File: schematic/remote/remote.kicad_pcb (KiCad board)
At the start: 2 copper layers, 14 parts, among them J1 Conn_01x05_Male, J2 Joystick_Left, J3 Joystick_Right, J4 Micro-Power-IN, J5 NRF-Power, U1 ARDUINO_PRO_MINI

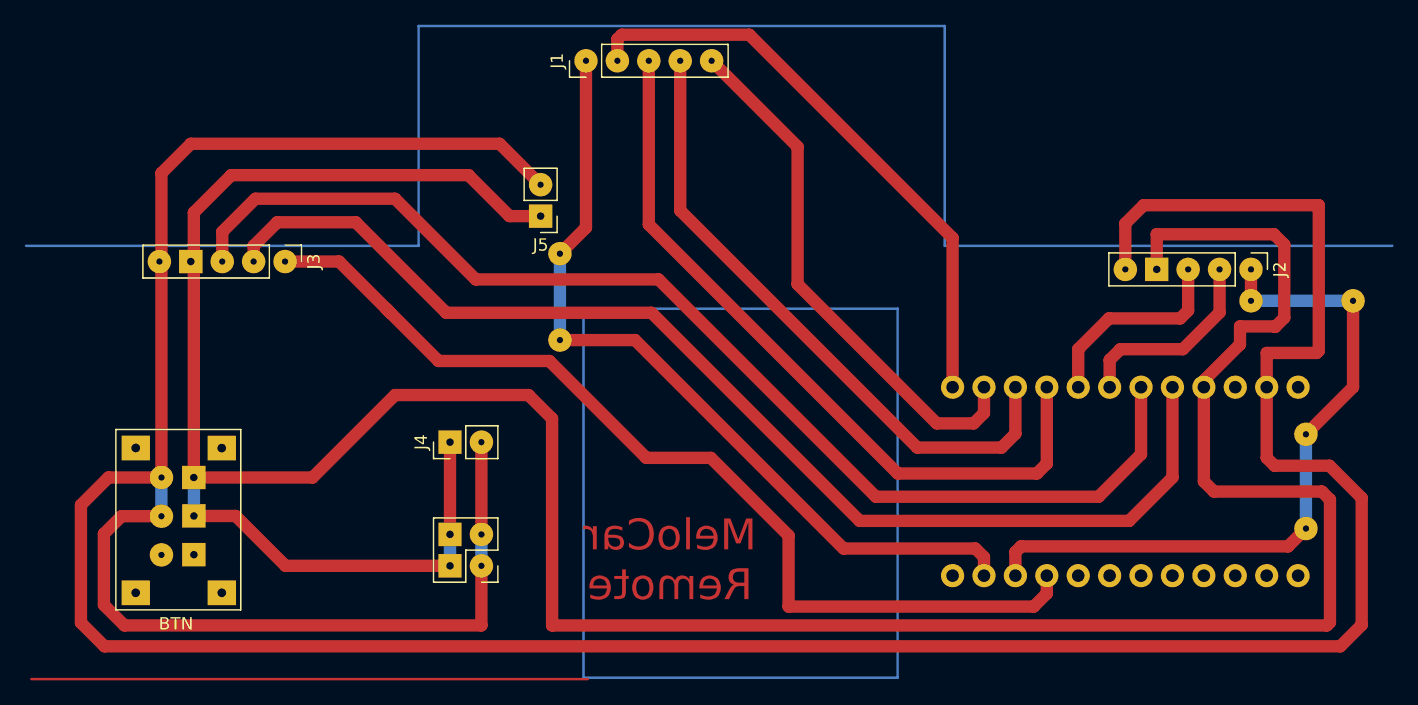
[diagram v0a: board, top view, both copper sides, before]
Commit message: e
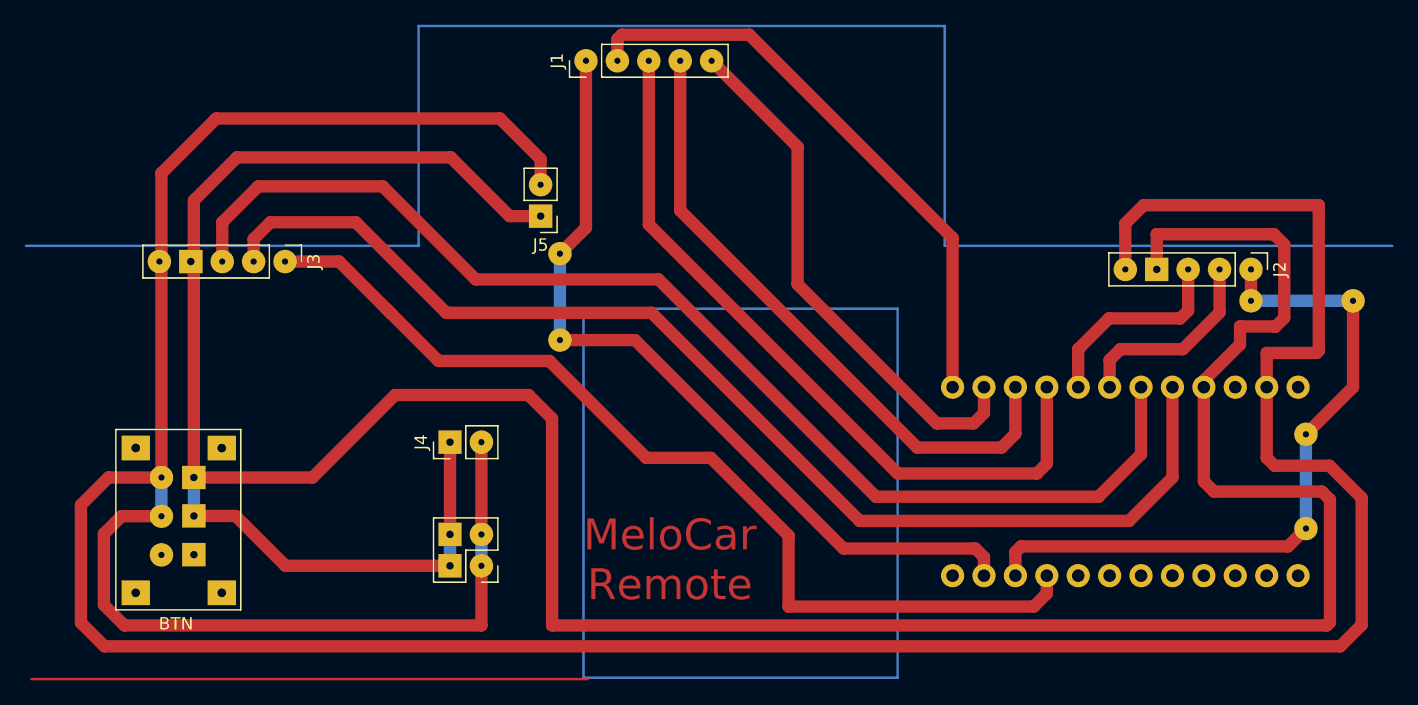
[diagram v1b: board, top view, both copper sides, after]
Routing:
- net GND: track 303.6 -> 306.5 mm
- net +5V: track 257.7 -> 259.4 mm
- net Net-(U1-PadJP6_6): track 94.6 -> 95.9 mm
